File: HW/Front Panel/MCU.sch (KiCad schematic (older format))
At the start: 31 parts, among them J1 CTRL, J2 MODE, J3 I2C, J4 ICE, J5 CAL, J6 PWM_DUAL, J7 CTRL_IN, J8 SERIAL, U2 M0516LDN, U3 TJCTM24028-SPI, X1 XTAL

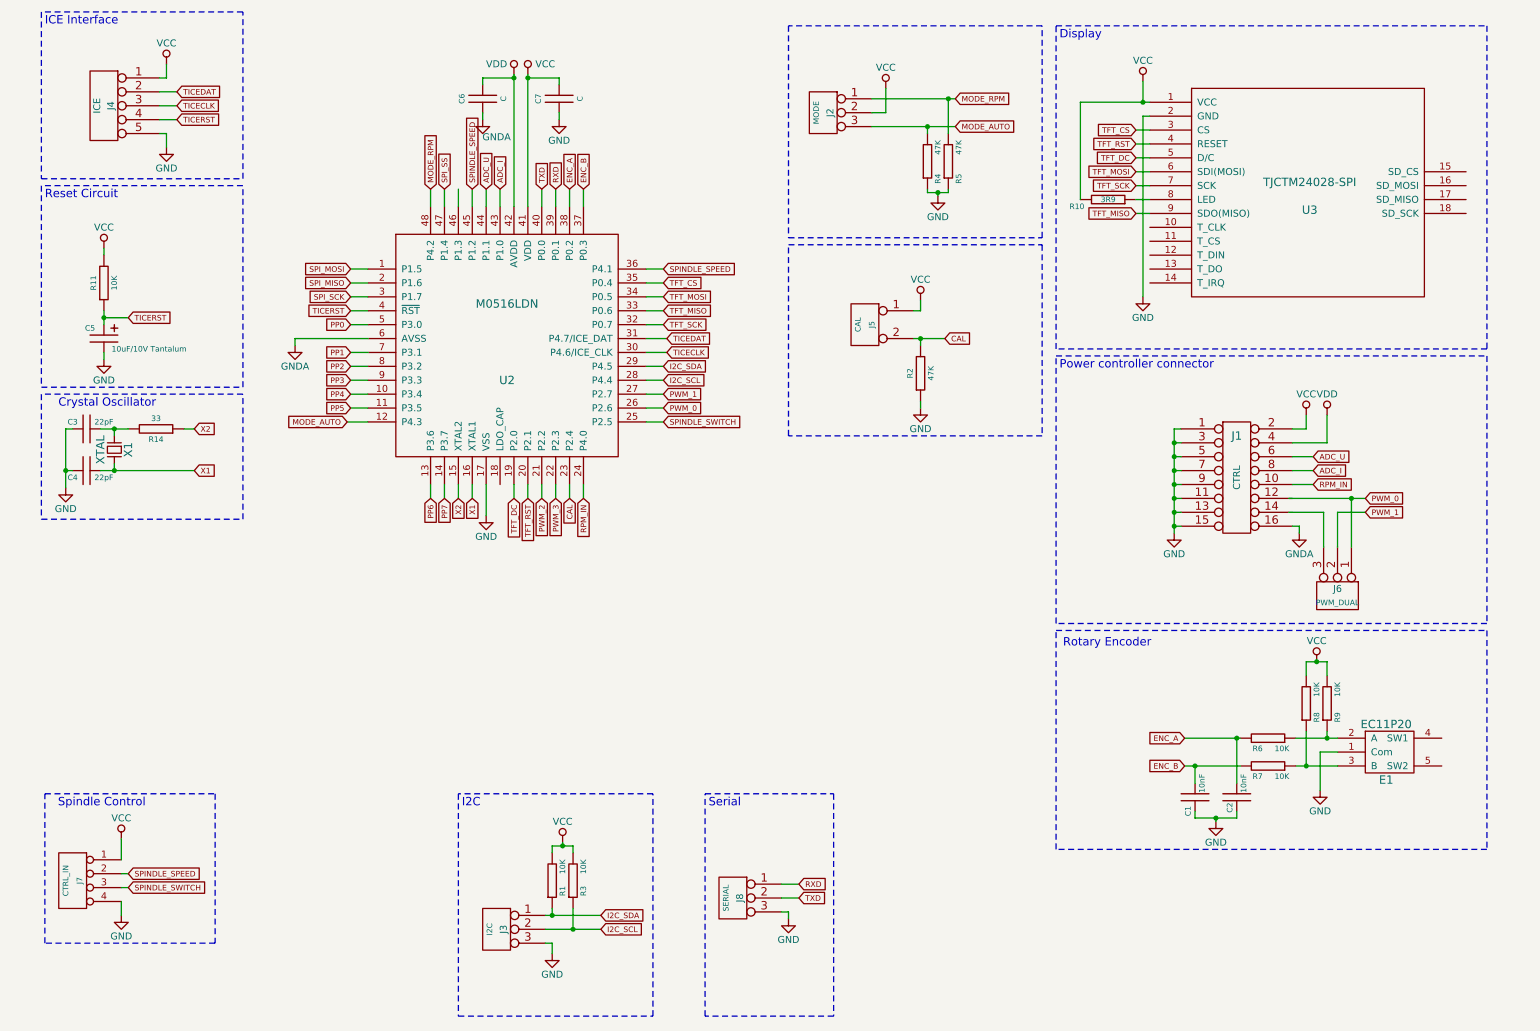
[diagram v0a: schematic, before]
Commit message: Before Front Panel next revision
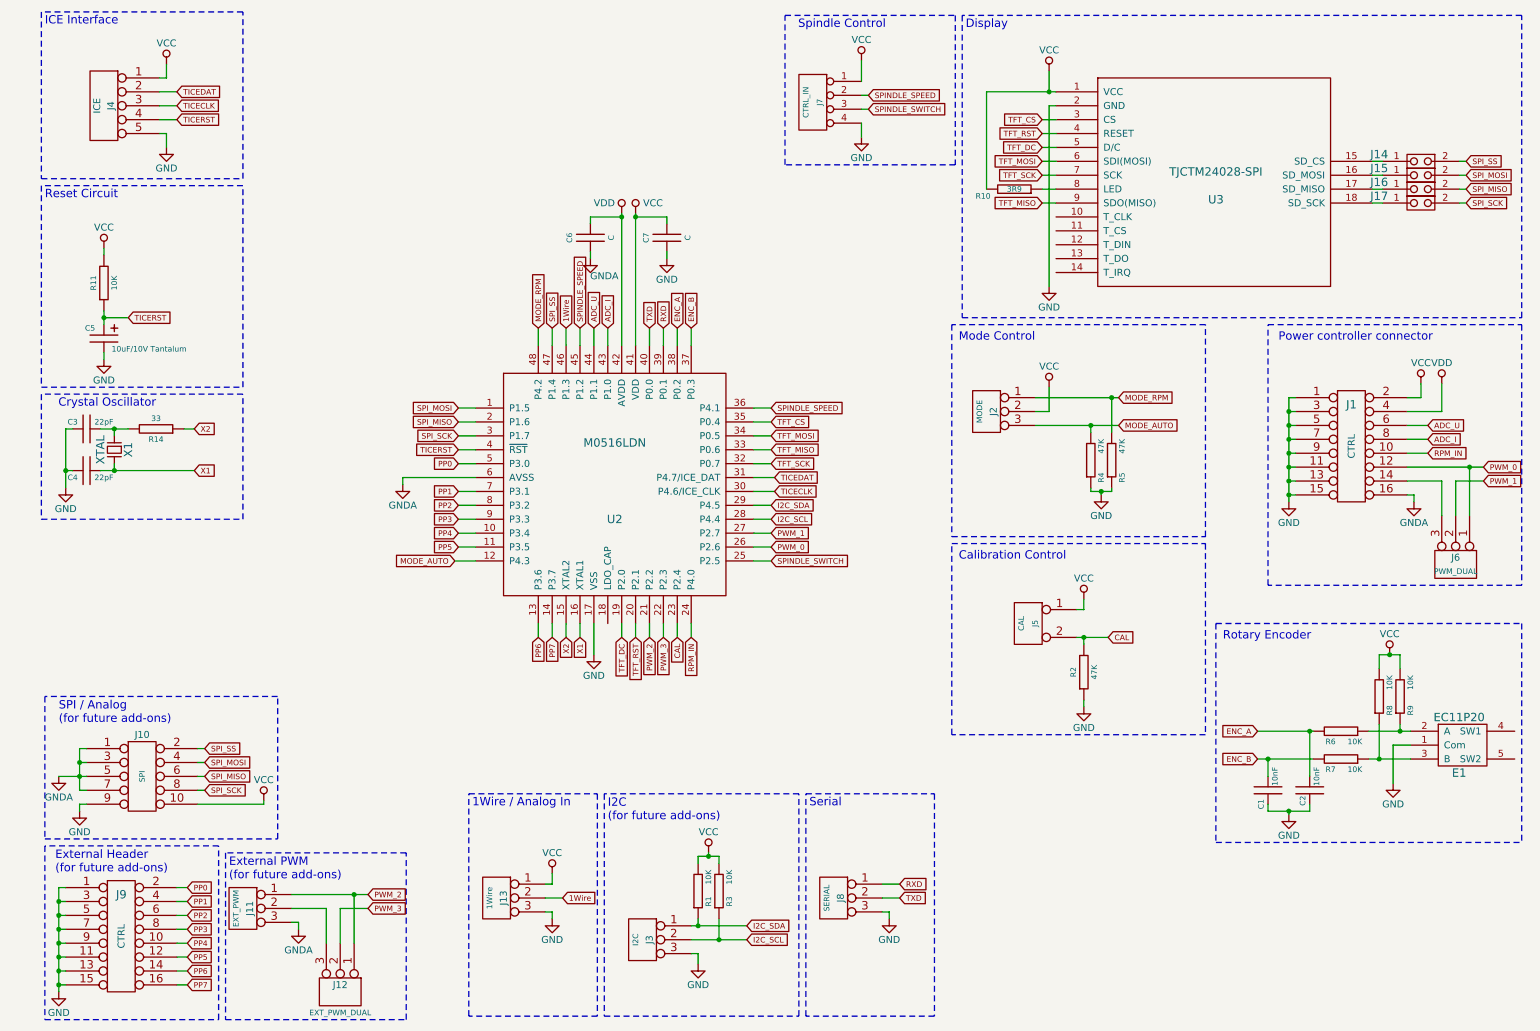
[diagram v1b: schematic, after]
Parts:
- added J10: SPI, Pin_Headers:Pin_Header_Straight_2x05, symbol CONN_5X2
- added J11: EXT_PWM, suf_connector_ncw:CONN_NCW254-03S, symbol CONN_3
- added J12: EXT_PWM_DUAL, Pin_Headers:Pin_Header_Straight_1x03, symbol CONN_3
- added J13: 1Wire, suf_connector_ncw:CONN_NCW254-03S, symbol CONN_3
- added J14, J15, J16, J17: JUMPER, Pin_Headers:Pin_Header_Straight_1x02, symbol JUMPER
- added J9: CTRL, Pin_Headers:Pin_Header_Straight_2x08, symbol CONN_8X2
- E1: footprint suf_switch:EC11P20_single_side -> suf_switch:EC11P20
- J4: footprint (none) -> Pin_Headers:Pin_Header_Straight_1x05
- J7: footprint suf_connector_ncw:CONN_NCW254-04S -> Pin_Headers:Pin_Header_Straight_1x04
- X1: footprint (none) -> Crystals:Crystal_HC49-SD_SMD
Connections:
- net GND: now also J10.9, J13.3 (P3), J9.1, J9.11, J9.13, J9.15, J9.3, J9.5, J9.7, J9.9
- net GNDA: now also J10.1, J10.3, J10.5, J10.7, J11.3 (P3)
- net PP0: now also J9.2
- net PP1: now also J9.4
- net PP2: now also J9.6
- net PP3: now also J9.8
- net PP4: now also J9.10
- net PP5: now also J9.12
- net PP6: now also J9.14
- net PP7: now also J9.16
- net PWM_0: now also J1.12
- net PWM_2: now also J11.1 (P1), J12.1 (P1)
- net PWM_3: now also J12.2 (PM)
- net SPI_MISO: now also J10.6, J16.2
- net SPI_MOSI: now also J10.4, J15.2
- net SPI_SCK: now also J10.8, J17.2
- net SPI_SS: now also J10.2, J14.2
- net VCC: now also J10.10, J13.1 (P1)
- net 1Wire: now reaches U2.46 (P1.3)
- net 1Wire: now also J13.2 (PM)
- net at U3.15 (SD_CS): now also J14.1
- net at U3.16 (SD_MOSI): now also J15.1
- net at U3.17 (SD_MISO): now also J16.1
- net at U3.18 (SD_SCK): now also J17.1
- net at J6.3 (P3): now also J1.14
- new net: J11.2 (PM), J12.3 (P3)
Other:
- note added: "1Wire / Analog In"
- note added: "Calibration Control"
- note added: "External Header\n(for future add-ons)"
- note added: "External PWM\n(for future add-ons)"
- note added: "I2C\n(for future add-ons)"
- note added: "Mode Control"
- note added: "SPI / Analog\n(for future add-ons)"
- note removed: "I2C"
- moved on the sheet: C1, C2, C6, C7, E1, J1, J2, J3, J5, J6, J7, J8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
